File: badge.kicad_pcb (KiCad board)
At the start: 2 copper layers, 100 x 100 mm, 1286 parts, among them IC1 SAMD21G18A-MU, J1 USB_C, J2 DEBUG, J3 LiPo 1S, SW1 A, SW2 B, SW3 X, SW4 Y, SW5 RESET, U1 IS31FL3236A, U2 IS31FL3236A, U3 GD25Q32C, U4 DW01, U5 AP2112K-3.3, U6 PM8205A, U7 HX4054A, X1 #badgelife

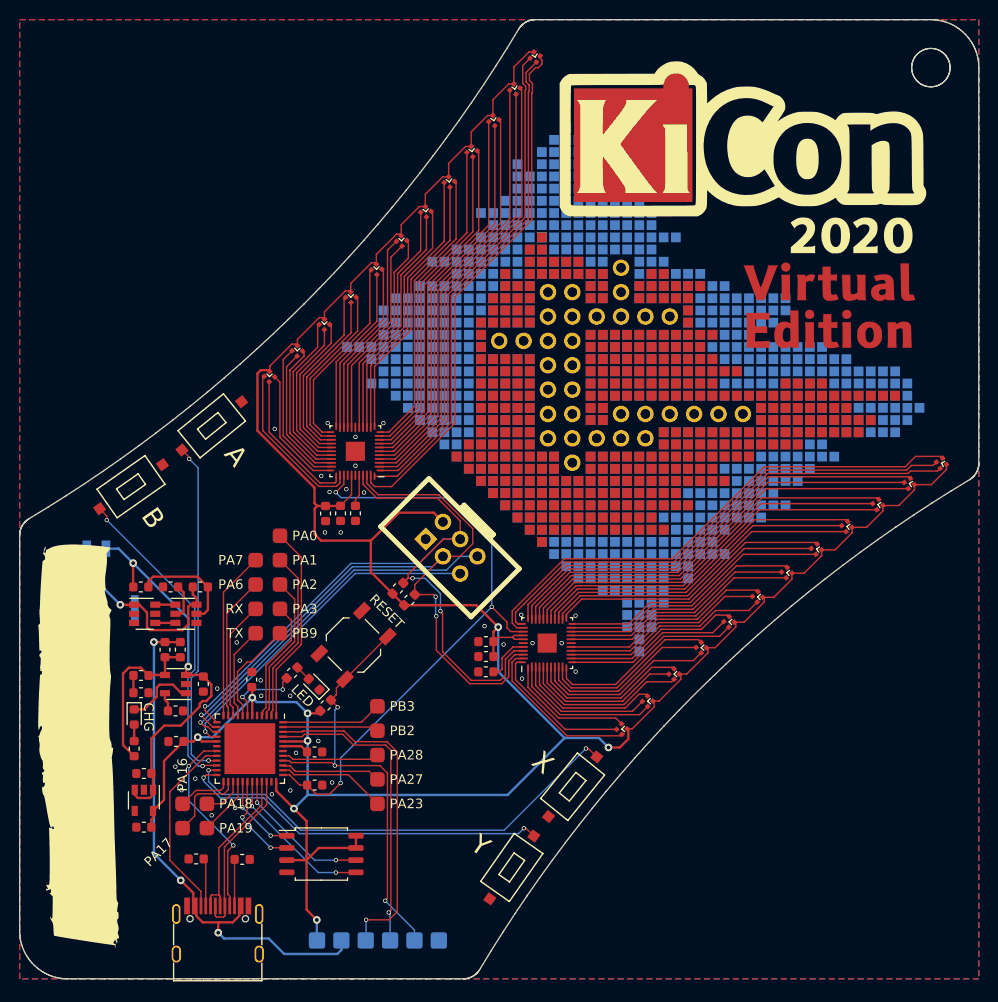
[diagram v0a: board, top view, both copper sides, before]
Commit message: gregdavill: Initial commit of new badge design
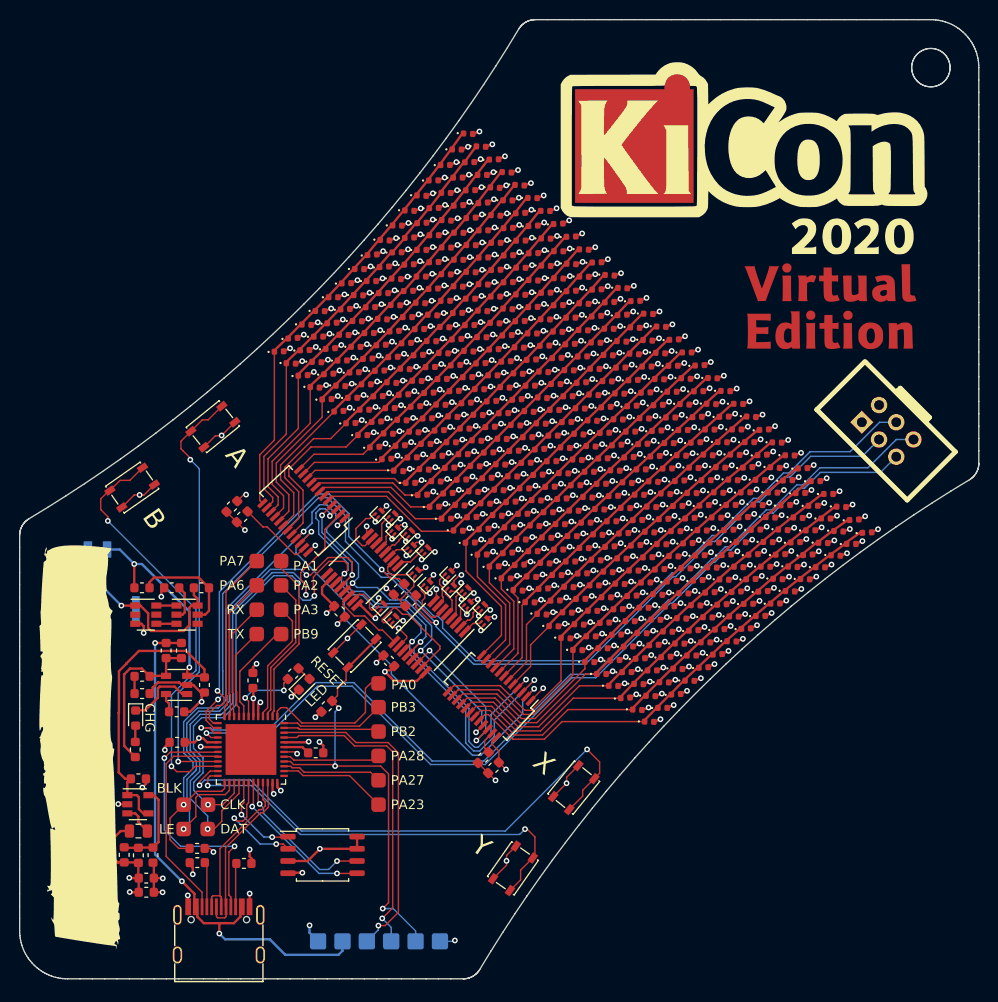
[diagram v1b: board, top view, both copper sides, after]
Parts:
- removed the R4 at (98.6, 118.0)
- removed REF** (x1161): Small_SMD_Proto_Pad, Connectors:Small_SMD_Proto_Pad
- removed REF** (x32): PTH_Proto_pad, Connectors:PTH_Proto_pad
- removed the TP1 at (77.1, 103.8)
- removed the U5 at (63.0, 131.4)
- added C13: 10uF, Capacitor_SMD:C_0603_1608Metric, F.Cu at (63.2, 141.0)
- added C14: 10uF, Capacitor_SMD:C_0603_1608Metric, F.Cu at (63.2, 139.5)
- added D100: LED, LED_SMD:LED_0402_1005Metric, F.Cu at (97.0, 70.7)
- added D101: LED, LED_SMD:LED_0402_1005Metric, F.Cu at (98.3, 72.0)
- added D102: LED, LED_SMD:LED_0402_1005Metric, F.Cu at (99.6, 73.3)
- added D103: LED, LED_SMD:LED_0402_1005Metric, F.Cu at (101.0, 74.6)
- added D104: LED, LED_SMD:LED_0402_1005Metric, F.Cu at (102.3, 75.9)
- added D105: LED, LED_SMD:LED_0402_1005Metric, F.Cu at (103.6, 77.2)
- added D106: LED, LED_SMD:LED_0402_1005Metric, F.Cu at (104.9, 78.5)
- added D107: LED, LED_SMD:LED_0402_1005Metric, F.Cu at (106.2, 79.8)
- added D108: LED, LED_SMD:LED_0402_1005Metric, F.Cu at (107.5, 81.1)
- added D109: LED, LED_SMD:LED_0402_1005Metric, F.Cu at (108.8, 82.4)
- added D110: LED, LED_SMD:LED_0402_1005Metric, F.Cu at (110.1, 83.7)
- added D111: LED, LED_SMD:LED_0402_1005Metric, F.Cu at (111.4, 85.0)
- added D112: LED, LED_SMD:LED_0402_1005Metric, F.Cu at (112.7, 86.3)
- added D113: LED, LED_SMD:LED_0402_1005Metric, F.Cu at (114.0, 87.6)
- added D114: LED, LED_SMD:LED_0402_1005Metric, F.Cu at (115.3, 88.9)
- added D115: LED, LED_SMD:LED_0402_1005Metric, F.Cu at (116.6, 90.2)
- added D116: LED, LED_SMD:LED_0402_1005Metric, F.Cu at (117.9, 91.5)
- added D117: LED, LED_SMD:LED_0402_1005Metric, F.Cu at (119.2, 92.8)
- added D118: LED, LED_SMD:LED_0402_1005Metric, F.Cu at (120.5, 94.1)
- added D119: LED, LED_SMD:LED_0402_1005Metric, F.Cu at (121.8, 95.4)
- added D120: LED, LED_SMD:LED_0402_1005Metric, F.Cu at (123.1, 96.7)
- added D121: LED, LED_SMD:LED_0402_1005Metric, F.Cu at (124.4, 98.0)
- added D122: LED, LED_SMD:LED_0402_1005Metric, F.Cu at (125.7, 99.3)
- added D123: LED, LED_SMD:LED_0402_1005Metric, F.Cu at (127.0, 100.6)
- added D124: LED, LED_SMD:LED_0402_1005Metric, F.Cu at (128.3, 101.9)
- added D125: LED, LED_SMD:LED_0402_1005Metric, F.Cu at (129.6, 103.2)
- added D126: LED, LED_SMD:LED_0402_1005Metric, F.Cu at (130.9, 104.5)
- added D127: LED, LED_SMD:LED_0402_1005Metric, F.Cu at (132.2, 105.8)
- added D128: LED, LED_SMD:LED_0402_1005Metric, F.Cu at (133.5, 107.1)
- added D129: LED, LED_SMD:LED_0402_1005Metric, F.Cu at (91.9, 68.3)
- added D130: LED, LED_SMD:LED_0402_1005Metric, F.Cu at (93.2, 69.6)
- added D131: LED, LED_SMD:LED_0402_1005Metric, F.Cu at (94.5, 70.9)
- added D132: LED, LED_SMD:LED_0402_1005Metric, F.Cu at (95.8, 72.2)
- added D133: LED, LED_SMD:LED_0402_1005Metric, F.Cu at (97.1, 73.5)
- added D134: LED, LED_SMD:LED_0402_1005Metric, F.Cu at (98.4, 74.8)
- added D135: LED, LED_SMD:LED_0402_1005Metric, F.Cu at (99.6, 76.1)
- added D136: LED, LED_SMD:LED_0402_1005Metric, F.Cu at (100.9, 77.4)
- added D137: LED, LED_SMD:LED_0402_1005Metric, F.Cu at (102.2, 78.7)
- added D138: LED, LED_SMD:LED_0402_1005Metric, F.Cu at (103.5, 80.0)
- added D139: LED, LED_SMD:LED_0402_1005Metric, F.Cu at (104.8, 81.2)
- added D140: LED, LED_SMD:LED_0402_1005Metric, F.Cu at (106.1, 82.5)
- added D141: LED, LED_SMD:LED_0402_1005Metric, F.Cu at (107.4, 83.8)
- added D142: LED, LED_SMD:LED_0402_1005Metric, F.Cu at (108.7, 85.1)
- added D143: LED, LED_SMD:LED_0402_1005Metric, F.Cu at (110.0, 86.4)
- added D144: LED, LED_SMD:LED_0402_1005Metric, F.Cu at (111.3, 87.7)
- added D145: LED, LED_SMD:LED_0402_1005Metric, F.Cu at (112.5, 89.0)
- added D146: LED, LED_SMD:LED_0402_1005Metric, F.Cu at (113.8, 90.3)
- added D147: LED, LED_SMD:LED_0402_1005Metric, F.Cu at (115.1, 91.6)
- added D148: LED, LED_SMD:LED_0402_1005Metric, F.Cu at (116.4, 92.9)
- added D149: LED, LED_SMD:LED_0402_1005Metric, F.Cu at (117.7, 94.1)
- added D150: LED, LED_SMD:LED_0402_1005Metric, F.Cu at (119.0, 95.4)
- added D151: LED, LED_SMD:LED_0402_1005Metric, F.Cu at (120.3, 96.7)
- added D152: LED, LED_SMD:LED_0402_1005Metric, F.Cu at (121.6, 98.0)
- added D153: LED, LED_SMD:LED_0402_1005Metric, F.Cu at (122.9, 99.3)
- added D154: LED, LED_SMD:LED_0402_1005Metric, F.Cu at (124.1, 100.6)
- added D155: LED, LED_SMD:LED_0402_1005Metric, F.Cu at (125.4, 101.9)
- added D156: LED, LED_SMD:LED_0402_1005Metric, F.Cu at (126.7, 103.2)
- added D157: LED, LED_SMD:LED_0402_1005Metric, F.Cu at (128.0, 104.5)
- added D158: LED, LED_SMD:LED_0402_1005Metric, F.Cu at (129.3, 105.8)
- added D159: LED, LED_SMD:LED_0402_1005Metric, F.Cu at (130.6, 107.0)
- added D160: LED, LED_SMD:LED_0402_1005Metric, F.Cu at (131.9, 108.3)
- added D161: LED, LED_SMD:LED_0402_1005Metric, F.Cu at (90.6, 69.9)
- added D162: LED, LED_SMD:LED_0402_1005Metric, F.Cu at (91.9, 71.2)
- added D163: LED, LED_SMD:LED_0402_1005Metric, F.Cu at (93.2, 72.5)
- added D164: LED, LED_SMD:LED_0402_1005Metric, F.Cu at (94.5, 73.8)
- added D165: LED, LED_SMD:LED_0402_1005Metric, F.Cu at (95.8, 75.0)
- added D166: LED, LED_SMD:LED_0402_1005Metric, F.Cu at (97.0, 76.3)
- added D167: LED, LED_SMD:LED_0402_1005Metric, F.Cu at (98.3, 77.6)
- added D168: LED, LED_SMD:LED_0402_1005Metric, F.Cu at (99.6, 78.9)
- added D169: LED, LED_SMD:LED_0402_1005Metric, F.Cu at (100.9, 80.2)
- added D170: LED, LED_SMD:LED_0402_1005Metric, F.Cu at (102.2, 81.4)
- added D171: LED, LED_SMD:LED_0402_1005Metric, F.Cu at (103.4, 82.7)
- added D172: LED, LED_SMD:LED_0402_1005Metric, F.Cu at (104.7, 84.0)
- added D173: LED, LED_SMD:LED_0402_1005Metric, F.Cu at (106.0, 85.3)
- added D174: LED, LED_SMD:LED_0402_1005Metric, F.Cu at (107.3, 86.6)
- added D175: LED, LED_SMD:LED_0402_1005Metric, F.Cu at (108.6, 87.8)
- added D176: LED, LED_SMD:LED_0402_1005Metric, F.Cu at (109.8, 89.1)
- added D177: LED, LED_SMD:LED_0402_1005Metric, F.Cu at (111.1, 90.4)
- added D178: LED, LED_SMD:LED_0402_1005Metric, F.Cu at (112.4, 91.7)
- added D179: LED, LED_SMD:LED_0402_1005Metric, F.Cu at (113.7, 93.0)
- added D180: LED, LED_SMD:LED_0402_1005Metric, F.Cu at (115.0, 94.2)
- added D181: LED, LED_SMD:LED_0402_1005Metric, F.Cu at (116.2, 95.5)
- added D182: LED, LED_SMD:LED_0402_1005Metric, F.Cu at (117.5, 96.8)
- added D183: LED, LED_SMD:LED_0402_1005Metric, F.Cu at (118.8, 98.1)
- added D184: LED, LED_SMD:LED_0402_1005Metric, F.Cu at (120.1, 99.4)
- added D185: LED, LED_SMD:LED_0402_1005Metric, F.Cu at (121.4, 100.6)
- added D186: LED, LED_SMD:LED_0402_1005Metric, F.Cu at (122.6, 101.9)
- added D187: LED, LED_SMD:LED_0402_1005Metric, F.Cu at (123.9, 103.2)
- added D188: LED, LED_SMD:LED_0402_1005Metric, F.Cu at (125.2, 104.5)
- added D189: LED, LED_SMD:LED_0402_1005Metric, F.Cu at (126.5, 105.8)
- added D190: LED, LED_SMD:LED_0402_1005Metric, F.Cu at (127.8, 107.0)
- added D191: LED, LED_SMD:LED_0402_1005Metric, F.Cu at (129.0, 108.3)
- added D192: LED, LED_SMD:LED_0402_1005Metric, F.Cu at (130.3, 109.6)
- added D193: LED, LED_SMD:LED_0402_1005Metric, F.Cu at (89.4, 71.5)
- added D194: LED, LED_SMD:LED_0402_1005Metric, F.Cu at (90.6, 72.7)
- added D195: LED, LED_SMD:LED_0402_1005Metric, F.Cu at (91.9, 74.0)
- added D196: LED, LED_SMD:LED_0402_1005Metric, F.Cu at (93.2, 75.3)
- added D197: LED, LED_SMD:LED_0402_1005Metric, F.Cu at (94.4, 76.5)
- added D198: LED, LED_SMD:LED_0402_1005Metric, F.Cu at (95.7, 77.8)
- added D199: LED, LED_SMD:LED_0402_1005Metric, F.Cu at (97.0, 79.1)
- added D200: LED, LED_SMD:LED_0402_1005Metric, F.Cu at (98.3, 80.4)
- added D201: LED, LED_SMD:LED_0402_1005Metric, F.Cu at (99.5, 81.6)
- added D202: LED, LED_SMD:LED_0402_1005Metric, F.Cu at (100.8, 82.9)
- added D203: LED, LED_SMD:LED_0402_1005Metric, F.Cu at (102.1, 84.2)
- added D204: LED, LED_SMD:LED_0402_1005Metric, F.Cu at (103.3, 85.4)
- added D205: LED, LED_SMD:LED_0402_1005Metric, F.Cu at (104.6, 86.7)
- added D206: LED, LED_SMD:LED_0402_1005Metric, F.Cu at (105.9, 88.0)
- added D207: LED, LED_SMD:LED_0402_1005Metric, F.Cu at (107.2, 89.3)
- added D208: LED, LED_SMD:LED_0402_1005Metric, F.Cu at (108.4, 90.5)
- added D209: LED, LED_SMD:LED_0402_1005Metric, F.Cu at (109.7, 91.8)
- added D210: LED, LED_SMD:LED_0402_1005Metric, F.Cu at (111.0, 93.1)
- added D211: LED, LED_SMD:LED_0402_1005Metric, F.Cu at (112.2, 94.3)
- added D212: LED, LED_SMD:LED_0402_1005Metric, F.Cu at (113.5, 95.6)
- added D213: LED, LED_SMD:LED_0402_1005Metric, F.Cu at (114.8, 96.9)
- added D214: LED, LED_SMD:LED_0402_1005Metric, F.Cu at (116.1, 98.2)
- added D215: LED, LED_SMD:LED_0402_1005Metric, F.Cu at (117.3, 99.4)
- added D216: LED, LED_SMD:LED_0402_1005Metric, F.Cu at (118.6, 100.7)
- added D217: LED, LED_SMD:LED_0402_1005Metric, F.Cu at (119.9, 102.0)
- added D218: LED, LED_SMD:LED_0402_1005Metric, F.Cu at (121.1, 103.2)
- added D219: LED, LED_SMD:LED_0402_1005Metric, F.Cu at (122.4, 104.5)
- added D220: LED, LED_SMD:LED_0402_1005Metric, F.Cu at (123.7, 105.8)
- added D221: LED, LED_SMD:LED_0402_1005Metric, F.Cu at (125.0, 107.1)
- added D222: LED, LED_SMD:LED_0402_1005Metric, F.Cu at (126.2, 108.3)
- added D223: LED, LED_SMD:LED_0402_1005Metric, F.Cu at (127.5, 109.6)
- added D224: LED, LED_SMD:LED_0402_1005Metric, F.Cu at (128.8, 110.9)
- added D225: LED, LED_SMD:LED_0402_1005Metric, F.Cu at (88.1, 73.0)
- added D226: LED, LED_SMD:LED_0402_1005Metric, F.Cu at (89.3, 74.3)
- added D227: LED, LED_SMD:LED_0402_1005Metric, F.Cu at (90.6, 75.5)
- added D228: LED, LED_SMD:LED_0402_1005Metric, F.Cu at (91.9, 76.8)
- added D229: LED, LED_SMD:LED_0402_1005Metric, F.Cu at (93.1, 78.1)
- added D230: LED, LED_SMD:LED_0402_1005Metric, F.Cu at (94.4, 79.3)
- added D231: LED, LED_SMD:LED_0402_1005Metric, F.Cu at (95.6, 80.6)
- added D232: LED, LED_SMD:LED_0402_1005Metric, F.Cu at (96.9, 81.8)
- added D233: LED, LED_SMD:LED_0402_1005Metric, F.Cu at (98.2, 83.1)
- added D234: LED, LED_SMD:LED_0402_1005Metric, F.Cu at (99.4, 84.4)
- added D235: LED, LED_SMD:LED_0402_1005Metric, F.Cu at (100.7, 85.6)
- added D236: LED, LED_SMD:LED_0402_1005Metric, F.Cu at (102.0, 86.9)
- added D237: LED, LED_SMD:LED_0402_1005Metric, F.Cu at (103.2, 88.2)
- added D238: LED, LED_SMD:LED_0402_1005Metric, F.Cu at (104.5, 89.4)
- added D239: LED, LED_SMD:LED_0402_1005Metric, F.Cu at (105.8, 90.7)
- added D240: LED, LED_SMD:LED_0402_1005Metric, F.Cu at (107.0, 92.0)
- added D241: LED, LED_SMD:LED_0402_1005Metric, F.Cu at (108.3, 93.2)
- added D242: LED, LED_SMD:LED_0402_1005Metric, F.Cu at (109.5, 94.5)
- added D243: LED, LED_SMD:LED_0402_1005Metric, F.Cu at (110.8, 95.7)
- added D244: LED, LED_SMD:LED_0402_1005Metric, F.Cu at (112.1, 97.0)
- added D245: LED, LED_SMD:LED_0402_1005Metric, F.Cu at (113.3, 98.3)
- added D246: LED, LED_SMD:LED_0402_1005Metric, F.Cu at (114.6, 99.5)
- added D247: LED, LED_SMD:LED_0402_1005Metric, F.Cu at (115.9, 100.8)
- added D248: LED, LED_SMD:LED_0402_1005Metric, F.Cu at (117.1, 102.1)
- added D249: LED, LED_SMD:LED_0402_1005Metric, F.Cu at (118.4, 103.3)
- added D25: LED, LED_SMD:LED_0402_1005Metric, F.Cu at (129.0, 94.1)
- added D250: LED, LED_SMD:LED_0402_1005Metric, F.Cu at (119.7, 104.6)
- added D251: LED, LED_SMD:LED_0402_1005Metric, F.Cu at (120.9, 105.9)
- added D252: LED, LED_SMD:LED_0402_1005Metric, F.Cu at (122.2, 107.1)
- added D253: LED, LED_SMD:LED_0402_1005Metric, F.Cu at (123.4, 108.4)
- added D254: LED, LED_SMD:LED_0402_1005Metric, F.Cu at (124.7, 109.6)
- added D255: LED, LED_SMD:LED_0402_1005Metric, F.Cu at (126.0, 110.9)
- added D256: LED, LED_SMD:LED_0402_1005Metric, F.Cu at (127.2, 112.2)
- added D257: LED, LED_SMD:LED_0402_1005Metric, F.Cu at (86.8, 74.5)
- added D258: LED, LED_SMD:LED_0402_1005Metric, F.Cu at (88.0, 75.8)
- added D259: LED, LED_SMD:LED_0402_1005Metric, F.Cu at (89.3, 77.0)
- added D26: LED, LED_SMD:LED_0402_1005Metric, F.Cu at (130.3, 95.4)
- added D260: LED, LED_SMD:LED_0402_1005Metric, F.Cu at (90.5, 78.3)
- added D261: LED, LED_SMD:LED_0402_1005Metric, F.Cu at (91.8, 79.5)
- added D262: LED, LED_SMD:LED_0402_1005Metric, F.Cu at (93.0, 80.8)
- added D263: LED, LED_SMD:LED_0402_1005Metric, F.Cu at (94.3, 82.1)
- added D264: LED, LED_SMD:LED_0402_1005Metric, F.Cu at (95.6, 83.3)
- added D265: LED, LED_SMD:LED_0402_1005Metric, F.Cu at (96.8, 84.6)
- added D266: LED, LED_SMD:LED_0402_1005Metric, F.Cu at (98.1, 85.8)
- added D267: LED, LED_SMD:LED_0402_1005Metric, F.Cu at (99.3, 87.1)
- added D268: LED, LED_SMD:LED_0402_1005Metric, F.Cu at (100.6, 88.3)
- added D269: LED, LED_SMD:LED_0402_1005Metric, F.Cu at (101.8, 89.6)
- added D27: LED, LED_SMD:LED_0402_1005Metric, F.Cu at (131.6, 96.8)
- added D270: LED, LED_SMD:LED_0402_1005Metric, F.Cu at (103.1, 90.9)
- added D271: LED, LED_SMD:LED_0402_1005Metric, F.Cu at (104.4, 92.1)
- added D272: LED, LED_SMD:LED_0402_1005Metric, F.Cu at (105.6, 93.4)
- added D273: LED, LED_SMD:LED_0402_1005Metric, F.Cu at (106.9, 94.6)
- added D274: LED, LED_SMD:LED_0402_1005Metric, F.Cu at (108.1, 95.9)
- added D275: LED, LED_SMD:LED_0402_1005Metric, F.Cu at (109.4, 97.1)
- added D276: LED, LED_SMD:LED_0402_1005Metric, F.Cu at (110.6, 98.4)
- added D277: LED, LED_SMD:LED_0402_1005Metric, F.Cu at (111.9, 99.7)
- added D278: LED, LED_SMD:LED_0402_1005Metric, F.Cu at (113.2, 100.9)
- added D279: LED, LED_SMD:LED_0402_1005Metric, F.Cu at (114.4, 102.2)
- added D28: LED, LED_SMD:LED_0402_1005Metric, F.Cu at (133.0, 98.1)
- added D280: LED, LED_SMD:LED_0402_1005Metric, F.Cu at (115.7, 103.4)
- added D281: LED, LED_SMD:LED_0402_1005Metric, F.Cu at (116.9, 104.7)
- added D282: LED, LED_SMD:LED_0402_1005Metric, F.Cu at (118.2, 105.9)
- added D283: LED, LED_SMD:LED_0402_1005Metric, F.Cu at (119.4, 107.2)
- added D284: LED, LED_SMD:LED_0402_1005Metric, F.Cu at (120.7, 108.5)
- added D285: LED, LED_SMD:LED_0402_1005Metric, F.Cu at (122.0, 109.7)
- added D286: LED, LED_SMD:LED_0402_1005Metric, F.Cu at (123.2, 111.0)
- added D287: LED, LED_SMD:LED_0402_1005Metric, F.Cu at (124.5, 112.2)
- added D288: LED, LED_SMD:LED_0402_1005Metric, F.Cu at (125.7, 113.5)
- added D289: LED, LED_SMD:LED_0402_1005Metric, F.Cu at (85.4, 76.0)
- added D29: LED, LED_SMD:LED_0402_1005Metric, F.Cu at (134.3, 99.5)
- added D290: LED, LED_SMD:LED_0402_1005Metric, F.Cu at (86.7, 77.3)
- added D291: LED, LED_SMD:LED_0402_1005Metric, F.Cu at (87.9, 78.5)
- added D292: LED, LED_SMD:LED_0402_1005Metric, F.Cu at (89.2, 79.8)
- added D293: LED, LED_SMD:LED_0402_1005Metric, F.Cu at (90.4, 81.0)
- added D294: LED, LED_SMD:LED_0402_1005Metric, F.Cu at (91.7, 82.3)
- added D295: LED, LED_SMD:LED_0402_1005Metric, F.Cu at (92.9, 83.5)
- added D296: LED, LED_SMD:LED_0402_1005Metric, F.Cu at (94.2, 84.8)
- added D297: LED, LED_SMD:LED_0402_1005Metric, F.Cu at (95.4, 86.0)
- added D298: LED, LED_SMD:LED_0402_1005Metric, F.Cu at (96.7, 87.3)
- added D299: LED, LED_SMD:LED_0402_1005Metric, F.Cu at (97.9, 88.5)
- added D30: LED, LED_SMD:LED_0402_1005Metric, F.Cu at (135.7, 100.8)
- added D300: LED, LED_SMD:LED_0402_1005Metric, F.Cu at (99.2, 89.8)
- added D301: LED, LED_SMD:LED_0402_1005Metric, F.Cu at (100.4, 91.0)
- added D302: LED, LED_SMD:LED_0402_1005Metric, F.Cu at (101.7, 92.3)
- added D303: LED, LED_SMD:LED_0402_1005Metric, F.Cu at (102.9, 93.5)
- added D304: LED, LED_SMD:LED_0402_1005Metric, F.Cu at (104.2, 94.8)
- added D305: LED, LED_SMD:LED_0402_1005Metric, F.Cu at (105.5, 96.0)
- added D306: LED, LED_SMD:LED_0402_1005Metric, F.Cu at (106.7, 97.3)
- added D307: LED, LED_SMD:LED_0402_1005Metric, F.Cu at (108.0, 98.5)
- added D308: LED, LED_SMD:LED_0402_1005Metric, F.Cu at (109.2, 99.8)
- added D309: LED, LED_SMD:LED_0402_1005Metric, F.Cu at (110.5, 101.0)
- added D31: LED, LED_SMD:LED_0402_1005Metric, F.Cu at (137.0, 102.1)
- added D310: LED, LED_SMD:LED_0402_1005Metric, F.Cu at (111.7, 102.3)
- added D311: LED, LED_SMD:LED_0402_1005Metric, F.Cu at (113.0, 103.5)
- added D312: LED, LED_SMD:LED_0402_1005Metric, F.Cu at (114.2, 104.8)
- added D313: LED, LED_SMD:LED_0402_1005Metric, F.Cu at (115.5, 106.1)
- added D314: LED, LED_SMD:LED_0402_1005Metric, F.Cu at (116.7, 107.3)
- added D315: LED, LED_SMD:LED_0402_1005Metric, F.Cu at (118.0, 108.6)
- added D316: LED, LED_SMD:LED_0402_1005Metric, F.Cu at (119.2, 109.8)
- added D317: LED, LED_SMD:LED_0402_1005Metric, F.Cu at (120.5, 111.1)
- added D318: LED, LED_SMD:LED_0402_1005Metric, F.Cu at (121.7, 112.3)
- added D319: LED, LED_SMD:LED_0402_1005Metric, F.Cu at (123.0, 113.6)
- added D32: LED, LED_SMD:LED_0402_1005Metric, F.Cu at (138.3, 103.5)
- added D320: LED, LED_SMD:LED_0402_1005Metric, F.Cu at (124.2, 114.8)
- added D321: LED, LED_SMD:LED_0402_1005Metric, F.Cu at (84.1, 77.5)
- added D322: LED, LED_SMD:LED_0402_1005Metric, F.Cu at (85.3, 78.7)
- added D323: LED, LED_SMD:LED_0402_1005Metric, F.Cu at (86.6, 80.0)
- added D324: LED, LED_SMD:LED_0402_1005Metric, F.Cu at (87.8, 81.2)
- added D325: LED, LED_SMD:LED_0402_1005Metric, F.Cu at (89.1, 82.5)
- added D326: LED, LED_SMD:LED_0402_1005Metric, F.Cu at (90.3, 83.7)
- added D327: LED, LED_SMD:LED_0402_1005Metric, F.Cu at (91.6, 85.0)
- added D328: LED, LED_SMD:LED_0402_1005Metric, F.Cu at (92.8, 86.2)
- added D329: LED, LED_SMD:LED_0402_1005Metric, F.Cu at (94.1, 87.5)
- added D33: LED, LED_SMD:LED_0402_1005Metric, F.Cu at (95.6, 63.5)
- added D330: LED, LED_SMD:LED_0402_1005Metric, F.Cu at (95.3, 88.7)
- added D331: LED, LED_SMD:LED_0402_1005Metric, F.Cu at (96.5, 90.0)
- added D332: LED, LED_SMD:LED_0402_1005Metric, F.Cu at (97.8, 91.2)
- added D333: LED, LED_SMD:LED_0402_1005Metric, F.Cu at (99.0, 92.5)
- added D334: LED, LED_SMD:LED_0402_1005Metric, F.Cu at (100.3, 93.7)
- added D335: LED, LED_SMD:LED_0402_1005Metric, F.Cu at (101.5, 95.0)
- added D336: LED, LED_SMD:LED_0402_1005Metric, F.Cu at (102.8, 96.2)
- added D337: LED, LED_SMD:LED_0402_1005Metric, F.Cu at (104.0, 97.4)
- added D338: LED, LED_SMD:LED_0402_1005Metric, F.Cu at (105.3, 98.7)
- added D339: LED, LED_SMD:LED_0402_1005Metric, F.Cu at (106.5, 99.9)
- added D34: LED, LED_SMD:LED_0402_1005Metric, F.Cu at (96.9, 64.9)
- added D340: LED, LED_SMD:LED_0402_1005Metric, F.Cu at (107.8, 101.2)
- added D341: LED, LED_SMD:LED_0402_1005Metric, F.Cu at (109.0, 102.4)
- added D342: LED, LED_SMD:LED_0402_1005Metric, F.Cu at (110.3, 103.7)
- added D343: LED, LED_SMD:LED_0402_1005Metric, F.Cu at (111.5, 104.9)
- added D344: LED, LED_SMD:LED_0402_1005Metric, F.Cu at (112.8, 106.2)
- added D345: LED, LED_SMD:LED_0402_1005Metric, F.Cu at (114.0, 107.4)
- added D346: LED, LED_SMD:LED_0402_1005Metric, F.Cu at (115.3, 108.7)
- added D347: LED, LED_SMD:LED_0402_1005Metric, F.Cu at (116.5, 109.9)
- added D348: LED, LED_SMD:LED_0402_1005Metric, F.Cu at (117.8, 111.2)
- added D349: LED, LED_SMD:LED_0402_1005Metric, F.Cu at (119.0, 112.4)
- added D35: LED, LED_SMD:LED_0402_1005Metric, F.Cu at (98.2, 66.2)
- added D350: LED, LED_SMD:LED_0402_1005Metric, F.Cu at (120.3, 113.7)
- added D351: LED, LED_SMD:LED_0402_1005Metric, F.Cu at (121.5, 114.9)
- added D352: LED, LED_SMD:LED_0402_1005Metric, F.Cu at (122.8, 116.2)
- added D353: LED, LED_SMD:LED_0402_1005Metric, F.Cu at (82.7, 78.9)
- added D354: LED, LED_SMD:LED_0402_1005Metric, F.Cu at (83.9, 80.2)
- added D355: LED, LED_SMD:LED_0402_1005Metric, F.Cu at (85.2, 81.4)
- added D356: LED, LED_SMD:LED_0402_1005Metric, F.Cu at (86.4, 82.7)
- added D357: LED, LED_SMD:LED_0402_1005Metric, F.Cu at (87.7, 83.9)
- added D358: LED, LED_SMD:LED_0402_1005Metric, F.Cu at (88.9, 85.2)
- added D359: LED, LED_SMD:LED_0402_1005Metric, F.Cu at (90.2, 86.4)
- added D36: LED, LED_SMD:LED_0402_1005Metric, F.Cu at (99.6, 67.5)
- added D360: LED, LED_SMD:LED_0402_1005Metric, F.Cu at (91.4, 87.7)
- added D361: LED, LED_SMD:LED_0402_1005Metric, F.Cu at (92.7, 88.9)
- added D362: LED, LED_SMD:LED_0402_1005Metric, F.Cu at (93.9, 90.1)
- added D363: LED, LED_SMD:LED_0402_1005Metric, F.Cu at (95.1, 91.4)
- added D364: LED, LED_SMD:LED_0402_1005Metric, F.Cu at (96.4, 92.6)
- added D365: LED, LED_SMD:LED_0402_1005Metric, F.Cu at (97.6, 93.9)
- added D366: LED, LED_SMD:LED_0402_1005Metric, F.Cu at (98.9, 95.1)
- added D367: LED, LED_SMD:LED_0402_1005Metric, F.Cu at (100.1, 96.4)
- added D368: LED, LED_SMD:LED_0402_1005Metric, F.Cu at (101.4, 97.6)
- added D369: LED, LED_SMD:LED_0402_1005Metric, F.Cu at (102.6, 98.9)
- added D37: LED, LED_SMD:LED_0402_1005Metric, F.Cu at (100.9, 68.8)
- added D370: LED, LED_SMD:LED_0402_1005Metric, F.Cu at (103.9, 100.1)
- added D371: LED, LED_SMD:LED_0402_1005Metric, F.Cu at (105.1, 101.4)
- added D372: LED, LED_SMD:LED_0402_1005Metric, F.Cu at (106.4, 102.6)
- added D373: LED, LED_SMD:LED_0402_1005Metric, F.Cu at (107.6, 103.8)
- added D374: LED, LED_SMD:LED_0402_1005Metric, F.Cu at (108.8, 105.1)
- added D375: LED, LED_SMD:LED_0402_1005Metric, F.Cu at (110.1, 106.3)
- added D376: LED, LED_SMD:LED_0402_1005Metric, F.Cu at (111.3, 107.6)
- added D377: LED, LED_SMD:LED_0402_1005Metric, F.Cu at (112.6, 108.8)
- added D378: LED, LED_SMD:LED_0402_1005Metric, F.Cu at (113.8, 110.1)
- added D379: LED, LED_SMD:LED_0402_1005Metric, F.Cu at (115.1, 111.3)
- added D38: LED, LED_SMD:LED_0402_1005Metric, F.Cu at (102.2, 70.2)
- added D380: LED, LED_SMD:LED_0402_1005Metric, F.Cu at (116.3, 112.6)
- added D381: LED, LED_SMD:LED_0402_1005Metric, F.Cu at (117.6, 113.8)
- added D382: LED, LED_SMD:LED_0402_1005Metric, F.Cu at (118.8, 115.0)
- added D383: LED, LED_SMD:LED_0402_1005Metric, F.Cu at (120.1, 116.3)
- added D384: LED, LED_SMD:LED_0402_1005Metric, F.Cu at (121.3, 117.5)
- added D385: LED, LED_SMD:LED_0402_1005Metric, F.Cu at (81.3, 80.4)
- added D386: LED, LED_SMD:LED_0402_1005Metric, F.Cu at (82.6, 81.6)
- added D387: LED, LED_SMD:LED_0402_1005Metric, F.Cu at (83.8, 82.9)
- added D388: LED, LED_SMD:LED_0402_1005Metric, F.Cu at (85.0, 84.1)
- added D389: LED, LED_SMD:LED_0402_1005Metric, F.Cu at (86.3, 85.4)
- added D39: LED, LED_SMD:LED_0402_1005Metric, F.Cu at (103.5, 71.5)
- added D390: LED, LED_SMD:LED_0402_1005Metric, F.Cu at (87.5, 86.6)
- added D391: LED, LED_SMD:LED_0402_1005Metric, F.Cu at (88.8, 87.8)
- added D392: LED, LED_SMD:LED_0402_1005Metric, F.Cu at (90.0, 89.1)
- added D393: LED, LED_SMD:LED_0402_1005Metric, F.Cu at (91.3, 90.3)
- added D394: LED, LED_SMD:LED_0402_1005Metric, F.Cu at (92.5, 91.6)
- added D395: LED, LED_SMD:LED_0402_1005Metric, F.Cu at (93.7, 92.8)
- added D396: LED, LED_SMD:LED_0402_1005Metric, F.Cu at (95.0, 94.1)
- added D397: LED, LED_SMD:LED_0402_1005Metric, F.Cu at (96.2, 95.3)
- added D398: LED, LED_SMD:LED_0402_1005Metric, F.Cu at (97.5, 96.5)
- added D399: LED, LED_SMD:LED_0402_1005Metric, F.Cu at (98.7, 97.8)
- added D40: LED, LED_SMD:LED_0402_1005Metric, F.Cu at (104.9, 72.8)
- added D400: LED, LED_SMD:LED_0402_1005Metric, F.Cu at (100.0, 99.0)
- added D401: LED, LED_SMD:LED_0402_1005Metric, F.Cu at (101.2, 100.3)
- added D402: LED, LED_SMD:LED_0402_1005Metric, F.Cu at (102.4, 101.5)
- added D403: LED, LED_SMD:LED_0402_1005Metric, F.Cu at (103.7, 102.8)
- added D404: LED, LED_SMD:LED_0402_1005Metric, F.Cu at (104.9, 104.0)
- added D405: LED, LED_SMD:LED_0402_1005Metric, F.Cu at (106.2, 105.2)
- added D406: LED, LED_SMD:LED_0402_1005Metric, F.Cu at (107.4, 106.5)
- added D407: LED, LED_SMD:LED_0402_1005Metric, F.Cu at (108.7, 107.7)
- added D408: LED, LED_SMD:LED_0402_1005Metric, F.Cu at (109.9, 109.0)
- added D409: LED, LED_SMD:LED_0402_1005Metric, F.Cu at (111.2, 110.2)
- added D41: LED, LED_SMD:LED_0402_1005Metric, F.Cu at (106.2, 74.1)
- added D410: LED, LED_SMD:LED_0402_1005Metric, F.Cu at (112.4, 111.5)
- added D411: LED, LED_SMD:LED_0402_1005Metric, F.Cu at (113.6, 112.7)
- added D412: LED, LED_SMD:LED_0402_1005Metric, F.Cu at (114.9, 114.0)
- added D413: LED, LED_SMD:LED_0402_1005Metric, F.Cu at (116.1, 115.2)
- added D414: LED, LED_SMD:LED_0402_1005Metric, F.Cu at (117.4, 116.4)
- added D415: LED, LED_SMD:LED_0402_1005Metric, F.Cu at (118.6, 117.7)
- added D416: LED, LED_SMD:LED_0402_1005Metric, F.Cu at (119.9, 118.9)
- added D417: LED, LED_SMD:LED_0402_1005Metric, F.Cu at (79.9, 81.8)
- added D418: LED, LED_SMD:LED_0402_1005Metric, F.Cu at (81.1, 83.0)
- added D419: LED, LED_SMD:LED_0402_1005Metric, F.Cu at (82.4, 84.3)
- added D42: LED, LED_SMD:LED_0402_1005Metric, F.Cu at (107.5, 75.5)
- added D420: LED, LED_SMD:LED_0402_1005Metric, F.Cu at (83.6, 85.5)
- added D421: LED, LED_SMD:LED_0402_1005Metric, F.Cu at (84.9, 86.8)
- added D422: LED, LED_SMD:LED_0402_1005Metric, F.Cu at (86.1, 88.0)
- added D423: LED, LED_SMD:LED_0402_1005Metric, F.Cu at (87.4, 89.3)
- added D424: LED, LED_SMD:LED_0402_1005Metric, F.Cu at (88.6, 90.5)
- added D425: LED, LED_SMD:LED_0402_1005Metric, F.Cu at (89.8, 91.7)
- added D426: LED, LED_SMD:LED_0402_1005Metric, F.Cu at (91.1, 93.0)
- added D427: LED, LED_SMD:LED_0402_1005Metric, F.Cu at (92.3, 94.2)
- added D428: LED, LED_SMD:LED_0402_1005Metric, F.Cu at (93.6, 95.5)
- added D429: LED, LED_SMD:LED_0402_1005Metric, F.Cu at (94.8, 96.7)
- added D43: LED, LED_SMD:LED_0402_1005Metric, F.Cu at (108.8, 76.8)
- added D430: LED, LED_SMD:LED_0402_1005Metric, F.Cu at (96.1, 98.0)
- added D431: LED, LED_SMD:LED_0402_1005Metric, F.Cu at (97.3, 99.2)
- added D432: LED, LED_SMD:LED_0402_1005Metric, F.Cu at (98.5, 100.4)
- added D433: LED, LED_SMD:LED_0402_1005Metric, F.Cu at (99.8, 101.7)
- added D434: LED, LED_SMD:LED_0402_1005Metric, F.Cu at (101.0, 102.9)
- added D435: LED, LED_SMD:LED_0402_1005Metric, F.Cu at (102.3, 104.2)
- added D436: LED, LED_SMD:LED_0402_1005Metric, F.Cu at (103.5, 105.4)
- added D437: LED, LED_SMD:LED_0402_1005Metric, F.Cu at (104.8, 106.7)
- added D438: LED, LED_SMD:LED_0402_1005Metric, F.Cu at (106.0, 107.9)
- added D439: LED, LED_SMD:LED_0402_1005Metric, F.Cu at (107.2, 109.1)
- added D44: LED, LED_SMD:LED_0402_1005Metric, F.Cu at (110.2, 78.1)
- added D440: LED, LED_SMD:LED_0402_1005Metric, F.Cu at (108.5, 110.4)
- added D441: LED, LED_SMD:LED_0402_1005Metric, F.Cu at (109.7, 111.6)
- added D442: LED, LED_SMD:LED_0402_1005Metric, F.Cu at (111.0, 112.9)
- added D443: LED, LED_SMD:LED_0402_1005Metric, F.Cu at (112.2, 114.1)
- added D444: LED, LED_SMD:LED_0402_1005Metric, F.Cu at (113.5, 115.4)
- added D445: LED, LED_SMD:LED_0402_1005Metric, F.Cu at (114.7, 116.6)
- added D446: LED, LED_SMD:LED_0402_1005Metric, F.Cu at (115.9, 117.8)
- added D447: LED, LED_SMD:LED_0402_1005Metric, F.Cu at (117.2, 119.1)
- added D448: LED, LED_SMD:LED_0402_1005Metric, F.Cu at (118.4, 120.3)
- added D449: LED, LED_SMD:LED_0402_1005Metric, F.Cu at (78.5, 83.2)
- added D45: LED, LED_SMD:LED_0402_1005Metric, F.Cu at (111.5, 79.5)
- added D450: LED, LED_SMD:LED_0402_1005Metric, F.Cu at (79.7, 84.5)
- added D451: LED, LED_SMD:LED_0402_1005Metric, F.Cu at (81.0, 85.7)
- added D452: LED, LED_SMD:LED_0402_1005Metric, F.Cu at (82.2, 86.9)
- added D453: LED, LED_SMD:LED_0402_1005Metric, F.Cu at (83.5, 88.2)
- added D454: LED, LED_SMD:LED_0402_1005Metric, F.Cu at (84.7, 89.4)
- added D455: LED, LED_SMD:LED_0402_1005Metric, F.Cu at (85.9, 90.7)
- added D456: LED, LED_SMD:LED_0402_1005Metric, F.Cu at (87.2, 91.9)
- added D457: LED, LED_SMD:LED_0402_1005Metric, F.Cu at (88.4, 93.2)
- added D458: LED, LED_SMD:LED_0402_1005Metric, F.Cu at (89.7, 94.4)
- added D459: LED, LED_SMD:LED_0402_1005Metric, F.Cu at (90.9, 95.6)
- added D46: LED, LED_SMD:LED_0402_1005Metric, F.Cu at (112.8, 80.8)
- added D460: LED, LED_SMD:LED_0402_1005Metric, F.Cu at (92.2, 96.9)
- added D461: LED, LED_SMD:LED_0402_1005Metric, F.Cu at (93.4, 98.1)
- added D462: LED, LED_SMD:LED_0402_1005Metric, F.Cu at (94.6, 99.4)
- added D463: LED, LED_SMD:LED_0402_1005Metric, F.Cu at (95.9, 100.6)
- added D464: LED, LED_SMD:LED_0402_1005Metric, F.Cu at (97.1, 101.9)
- added D465: LED, LED_SMD:LED_0402_1005Metric, F.Cu at (98.4, 103.1)
- added D466: LED, LED_SMD:LED_0402_1005Metric, F.Cu at (99.6, 104.3)
- added D467: LED, LED_SMD:LED_0402_1005Metric, F.Cu at (100.9, 105.6)
- added D468: LED, LED_SMD:LED_0402_1005Metric, F.Cu at (102.1, 106.8)
- added D469: LED, LED_SMD:LED_0402_1005Metric, F.Cu at (103.3, 108.1)
- added D47: LED, LED_SMD:LED_0402_1005Metric, F.Cu at (114.1, 82.1)
- added D470: LED, LED_SMD:LED_0402_1005Metric, F.Cu at (104.6, 109.3)
- added D471: LED, LED_SMD:LED_0402_1005Metric, F.Cu at (105.8, 110.6)
- added D472: LED, LED_SMD:LED_0402_1005Metric, F.Cu at (107.1, 111.8)
- added D473: LED, LED_SMD:LED_0402_1005Metric, F.Cu at (108.3, 113.1)
- added D474: LED, LED_SMD:LED_0402_1005Metric, F.Cu at (109.6, 114.3)
- added D475: LED, LED_SMD:LED_0402_1005Metric, F.Cu at (110.8, 115.5)
- added D476: LED, LED_SMD:LED_0402_1005Metric, F.Cu at (112.1, 116.8)
- added D477: LED, LED_SMD:LED_0402_1005Metric, F.Cu at (113.3, 118.0)
- added D478: LED, LED_SMD:LED_0402_1005Metric, F.Cu at (114.5, 119.3)
- added D479: LED, LED_SMD:LED_0402_1005Metric, F.Cu at (115.8, 120.5)
- added D48: LED, LED_SMD:LED_0402_1005Metric, F.Cu at (115.5, 83.4)
- added D480: LED, LED_SMD:LED_0402_1005Metric, F.Cu at (117.0, 121.8)
- added D481: LED, LED_SMD:LED_0402_1005Metric, F.Cu at (77.0, 84.6)
- added D482: LED, LED_SMD:LED_0402_1005Metric, F.Cu at (78.3, 85.8)
- added D483: LED, LED_SMD:LED_0402_1005Metric, F.Cu at (79.5, 87.1)
- added D484: LED, LED_SMD:LED_0402_1005Metric, F.Cu at (80.8, 88.3)
- added D485: LED, LED_SMD:LED_0402_1005Metric, F.Cu at (82.0, 89.6)
- added D486: LED, LED_SMD:LED_0402_1005Metric, F.Cu at (83.3, 90.8)
- added D487: LED, LED_SMD:LED_0402_1005Metric, F.Cu at (84.5, 92.1)
- added D488: LED, LED_SMD:LED_0402_1005Metric, F.Cu at (85.8, 93.3)
- added D489: LED, LED_SMD:LED_0402_1005Metric, F.Cu at (87.0, 94.6)
- added D49: LED, LED_SMD:LED_0402_1005Metric, F.Cu at (116.8, 84.8)
- added D490: LED, LED_SMD:LED_0402_1005Metric, F.Cu at (88.2, 95.8)
- added D491: LED, LED_SMD:LED_0402_1005Metric, F.Cu at (89.5, 97.0)
- added D492: LED, LED_SMD:LED_0402_1005Metric, F.Cu at (90.7, 98.3)
- added D493: LED, LED_SMD:LED_0402_1005Metric, F.Cu at (92.0, 99.5)
- added D494: LED, LED_SMD:LED_0402_1005Metric, F.Cu at (93.2, 100.8)
- added D495: LED, LED_SMD:LED_0402_1005Metric, F.Cu at (94.5, 102.0)
- added D496: LED, LED_SMD:LED_0402_1005Metric, F.Cu at (95.7, 103.3)
- added D497: LED, LED_SMD:LED_0402_1005Metric, F.Cu at (97.0, 104.5)
- added D498: LED, LED_SMD:LED_0402_1005Metric, F.Cu at (98.2, 105.8)
- added D499: LED, LED_SMD:LED_0402_1005Metric, F.Cu at (99.5, 107.0)
- added D50: LED, LED_SMD:LED_0402_1005Metric, F.Cu at (118.1, 86.1)
- added D500: LED, LED_SMD:LED_0402_1005Metric, F.Cu at (100.7, 108.3)
- added D501: LED, LED_SMD:LED_0402_1005Metric, F.Cu at (101.9, 109.5)
- added D502: LED, LED_SMD:LED_0402_1005Metric, F.Cu at (103.2, 110.7)
- added D503: LED, LED_SMD:LED_0402_1005Metric, F.Cu at (104.4, 112.0)
- added D504: LED, LED_SMD:LED_0402_1005Metric, F.Cu at (105.7, 113.2)
- added D505: LED, LED_SMD:LED_0402_1005Metric, F.Cu at (106.9, 114.5)
- added D506: LED, LED_SMD:LED_0402_1005Metric, F.Cu at (108.2, 115.7)
- added D507: LED, LED_SMD:LED_0402_1005Metric, F.Cu at (109.4, 117.0)
- added D508: LED, LED_SMD:LED_0402_1005Metric, F.Cu at (110.7, 118.2)
- added D509: LED, LED_SMD:LED_0402_1005Metric, F.Cu at (111.9, 119.5)
- added D51: LED, LED_SMD:LED_0402_1005Metric, F.Cu at (119.5, 87.4)
- added D510: LED, LED_SMD:LED_0402_1005Metric, F.Cu at (113.1, 120.7)
- added D511: LED, LED_SMD:LED_0402_1005Metric, F.Cu at (114.4, 122.0)
- added D512: LED, LED_SMD:LED_0402_1005Metric, F.Cu at (115.6, 123.2)
- added D52: LED, LED_SMD:LED_0402_1005Metric, F.Cu at (120.8, 88.7)
- added D53: LED, LED_SMD:LED_0402_1005Metric, F.Cu at (122.1, 90.1)
- added D54: LED, LED_SMD:LED_0402_1005Metric, F.Cu at (123.4, 91.4)
- added D55: LED, LED_SMD:LED_0402_1005Metric, F.Cu at (124.8, 92.7)
- added D56: LED, LED_SMD:LED_0402_1005Metric, F.Cu at (126.1, 94.0)
- added D57: LED, LED_SMD:LED_0402_1005Metric, F.Cu at (127.4, 95.4)
- added D58: LED, LED_SMD:LED_0402_1005Metric, F.Cu at (128.7, 96.7)
- added D59: LED, LED_SMD:LED_0402_1005Metric, F.Cu at (130.1, 98.0)
- added D60: LED, LED_SMD:LED_0402_1005Metric, F.Cu at (131.4, 99.4)
- added D61: LED, LED_SMD:LED_0402_1005Metric, F.Cu at (132.7, 100.7)
- added D62: LED, LED_SMD:LED_0402_1005Metric, F.Cu at (134.0, 102.0)
- added D63: LED, LED_SMD:LED_0402_1005Metric, F.Cu at (135.4, 103.3)
- added D64: LED, LED_SMD:LED_0402_1005Metric, F.Cu at (136.7, 104.7)
- added D65: LED, LED_SMD:LED_0402_1005Metric, F.Cu at (94.4, 65.2)
- added D66: LED, LED_SMD:LED_0402_1005Metric, F.Cu at (95.7, 66.5)
- added D67: LED, LED_SMD:LED_0402_1005Metric, F.Cu at (97.0, 67.8)
- added D68: LED, LED_SMD:LED_0402_1005Metric, F.Cu at (98.3, 69.1)
- added D69: LED, LED_SMD:LED_0402_1005Metric, F.Cu at (99.6, 70.4)
- added D70: LED, LED_SMD:LED_0402_1005Metric, F.Cu at (100.9, 71.7)
- added D71: LED, LED_SMD:LED_0402_1005Metric, F.Cu at (102.2, 73.0)
- added D72: LED, LED_SMD:LED_0402_1005Metric, F.Cu at (103.6, 74.3)
- added D73: LED, LED_SMD:LED_0402_1005Metric, F.Cu at (104.9, 75.7)
- added D74: LED, LED_SMD:LED_0402_1005Metric, F.Cu at (106.2, 77.0)
- added D75: LED, LED_SMD:LED_0402_1005Metric, F.Cu at (107.5, 78.3)
- added D76: LED, LED_SMD:LED_0402_1005Metric, F.Cu at (108.8, 79.6)
- added D77: LED, LED_SMD:LED_0402_1005Metric, F.Cu at (110.1, 80.9)
- added D78: LED, LED_SMD:LED_0402_1005Metric, F.Cu at (111.4, 82.2)
- added D79: LED, LED_SMD:LED_0402_1005Metric, F.Cu at (112.8, 83.5)
- added D80: LED, LED_SMD:LED_0402_1005Metric, F.Cu at (114.1, 84.9)
- added D81: LED, LED_SMD:LED_0402_1005Metric, F.Cu at (115.4, 86.2)
- added D82: LED, LED_SMD:LED_0402_1005Metric, F.Cu at (116.7, 87.5)
- added D83: LED, LED_SMD:LED_0402_1005Metric, F.Cu at (118.0, 88.8)
- added D84: LED, LED_SMD:LED_0402_1005Metric, F.Cu at (119.3, 90.1)
- added D85: LED, LED_SMD:LED_0402_1005Metric, F.Cu at (120.6, 91.4)
- added D86: LED, LED_SMD:LED_0402_1005Metric, F.Cu at (121.9, 92.7)
- added D87: LED, LED_SMD:LED_0402_1005Metric, F.Cu at (123.3, 94.0)
- added D88: LED, LED_SMD:LED_0402_1005Metric, F.Cu at (124.6, 95.4)
- added D89: LED, LED_SMD:LED_0402_1005Metric, F.Cu at (125.9, 96.7)
- added D90: LED, LED_SMD:LED_0402_1005Metric, F.Cu at (127.2, 98.0)
- added D91: LED, LED_SMD:LED_0402_1005Metric, F.Cu at (128.5, 99.3)
- added D92: LED, LED_SMD:LED_0402_1005Metric, F.Cu at (129.8, 100.6)
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- renumbered D25 to D513, D26 to D514, R12 to R10, R13 to R11, R14 to R12, R15 to R13, R16 to R14, R17 to R15, R18 to R16, R5 to R3, R6 to R4, R7 to R5, R8 to R6, R9 to R7, R10 to R8, TP17 to TP1, TP8 to TP10, TP9 to TP11, TP10 to TP12, TP11 to TP13, TP12 to TP14, TP18 to TP2, TP2 to TP4, TP3 to TP5, TP4 to TP6, TP5 to TP7, TP6 to TP8, TP7 to TP9, U3 to U5, U4 to U6, U6 to U8, U7 to U9
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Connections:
- C10 pad 1: VCC -> Net-(C10-Pad1)
- C10 pad 2: GND -> VCC
- C9 pad 1: /1s LiPo/BATT_PLUS -> GND
- C9 pad 2: GND -> /1s LiPo/BATT_PLUS
- D1 pad 1: VCC -> COL_GA0
- D1 pad 2: Net-(D1-Pad2) -> /ISSI 12 RGB A/COM_6
- D10 pad 1: VCC -> COL_GA9
- D10 pad 2: Net-(D10-Pad2) -> /ISSI 12 RGB A/COM_6
- D11 pad 1: VCC -> COL_GA10
- D11 pad 2: Net-(D11-Pad2) -> /ISSI 12 RGB A/COM_6
- D12 pad 1: VCC -> COL_GA11
- D12 pad 2: Net-(D12-Pad2) -> /ISSI 12 RGB A/COM_6
- D13 pad 1: VCC -> COL_GA12
- D13 pad 2: Net-(D13-Pad2) -> /ISSI 12 RGB A/COM_6
- D14 pad 1: VCC -> COL_GA13
- D14 pad 2: Net-(D14-Pad2) -> /ISSI 12 RGB A/COM_6
- D15 pad 1: VCC -> COL_GA14
- D15 pad 2: Net-(D15-Pad2) -> /ISSI 12 RGB A/COM_6
- D16 pad 1: VCC -> COL_GA15
- D16 pad 2: Net-(D16-Pad2) -> /ISSI 12 RGB A/COM_6
- D17 pad 1: VCC -> COL_GA16
- D17 pad 2: Net-(D17-Pad2) -> /ISSI 12 RGB A/COM_6
- D18 pad 1: VCC -> COL_GA17
- D18 pad 2: Net-(D18-Pad2) -> /ISSI 12 RGB A/COM_6
- D19 pad 1: VCC -> COL_GA18
- D19 pad 2: Net-(D19-Pad2) -> /ISSI 12 RGB A/COM_6
- D2 pad 1: VCC -> COL_GA1
- D2 pad 2: Net-(D2-Pad2) -> /ISSI 12 RGB A/COM_6
- D20 pad 1: VCC -> COL_GA19
- D20 pad 2: Net-(D20-Pad2) -> /ISSI 12 RGB A/COM_6
- D21 pad 1: VCC -> COL_GA20
- D21 pad 2: Net-(D21-Pad2) -> /ISSI 12 RGB A/COM_6
- D22 pad 1: VCC -> COL_GA21
- D22 pad 2: Net-(D22-Pad2) -> /ISSI 12 RGB A/COM_6
- D23 pad 1: VCC -> COL_GA22
- D23 pad 2: Net-(D23-Pad2) -> /ISSI 12 RGB A/COM_6
- D24 pad 1: VCC -> COL_GA23
- D24 pad 2: Net-(D24-Pad2) -> /ISSI 12 RGB A/COM_6
- D3 pad 1: VCC -> COL_GA2
- D3 pad 2: Net-(D3-Pad2) -> /ISSI 12 RGB A/COM_6
- D4 pad 1: VCC -> COL_GA3
- D4 pad 2: Net-(D4-Pad2) -> /ISSI 12 RGB A/COM_6
- D5 pad 1: VCC -> COL_GA4
- D5 pad 2: Net-(D5-Pad2) -> /ISSI 12 RGB A/COM_6
- D6 pad 1: VCC -> COL_GA5
- D6 pad 2: Net-(D6-Pad2) -> /ISSI 12 RGB A/COM_6
- D7 pad 1: VCC -> COL_GA6
- D7 pad 2: Net-(D7-Pad2) -> /ISSI 12 RGB A/COM_6
- D8 pad 1: VCC -> COL_GA7
- D8 pad 2: Net-(D8-Pad2) -> /ISSI 12 RGB A/COM_6
- D9 pad 1: VCC -> COL_GA8
- D9 pad 2: Net-(D9-Pad2) -> /ISSI 12 RGB A/COM_6
- IC1 pad 25: Net-(IC1-Pad25) -> /LED_BLANK
- IC1 pad 26: Net-(IC1-Pad26) -> /LED_LATCH
- IC1 pad 27: Net-(IC1-Pad27) -> /LED_SCLK
- IC1 pad 28: Net-(IC1-Pad28) -> /LED_DAT
- IC1 pad 37: /SDB -> (no net)
- R9 pad 1: GND -> VCC
- R9 pad 2: /SDB -> /LED_BLANK
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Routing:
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- added copper zone on In2.Cu, net GND
- added copper zone on In1.Cu, net VCC
- removed copper zone on B.Cu, net GND
- removed copper zone on F.Cu, net GND
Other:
- copper layers 2 -> 4
- board text added: "@gregdavill"
- board text added: "BLK"
- board text added: "CLK"
- board text added: "DAT"
- board text added: "LE"
- board text removed: "PA16"
- board text removed: "PA17"
- board text removed: "PA18"
- board text removed: "PA19"
